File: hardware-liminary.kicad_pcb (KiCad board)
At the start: 2 copper layers, 149.2 x 73 mm, 55 parts, among them IC1 MCP6001T-I_OT, J3 UFL-Conn, J4 SWD, J5 Console, J6 Nema 7-Pin, K1 HL2-1CH-12S, Q1 CMBT2222A, Q2 PT204-6C, Q3 CMBT3904, SW1 SW_Push, U1 EESAMR34J18-V1_CT, U2 LD1117S33TR_SOT223

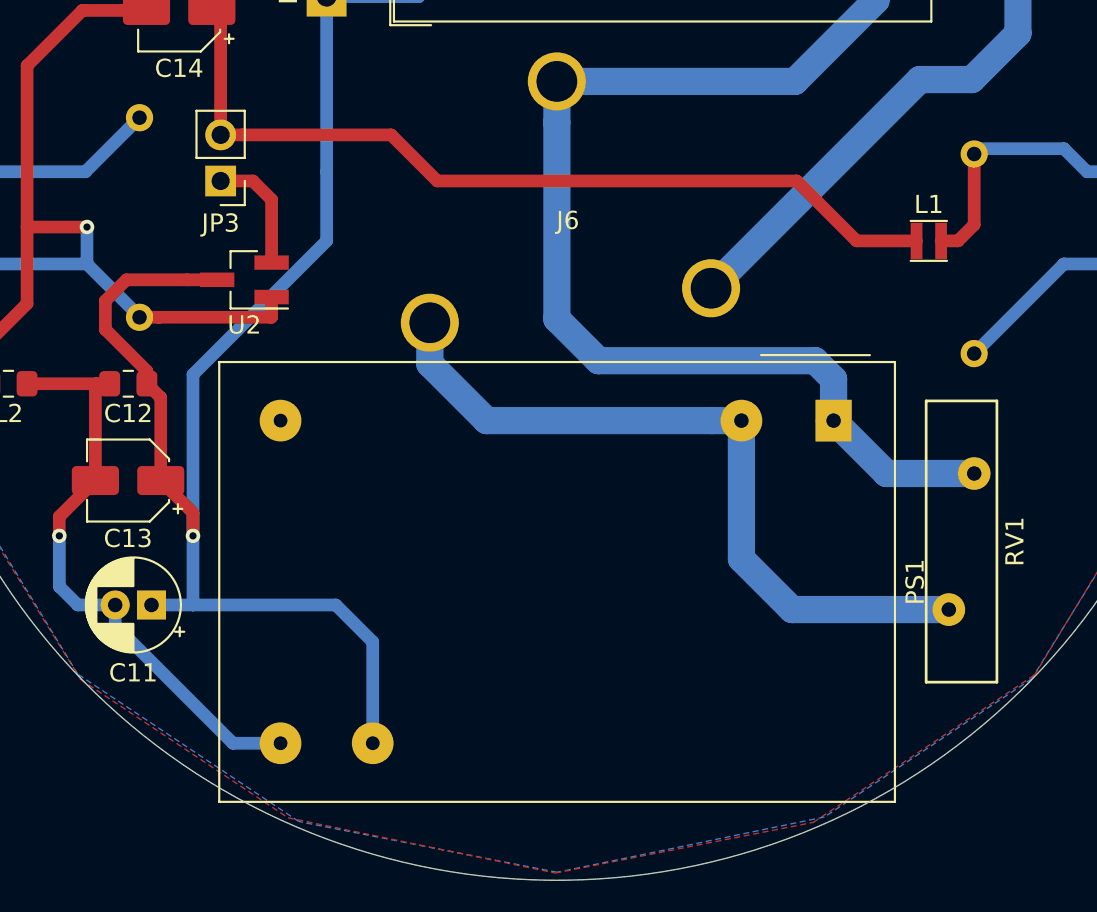
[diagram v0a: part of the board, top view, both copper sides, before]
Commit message: Correciones menores
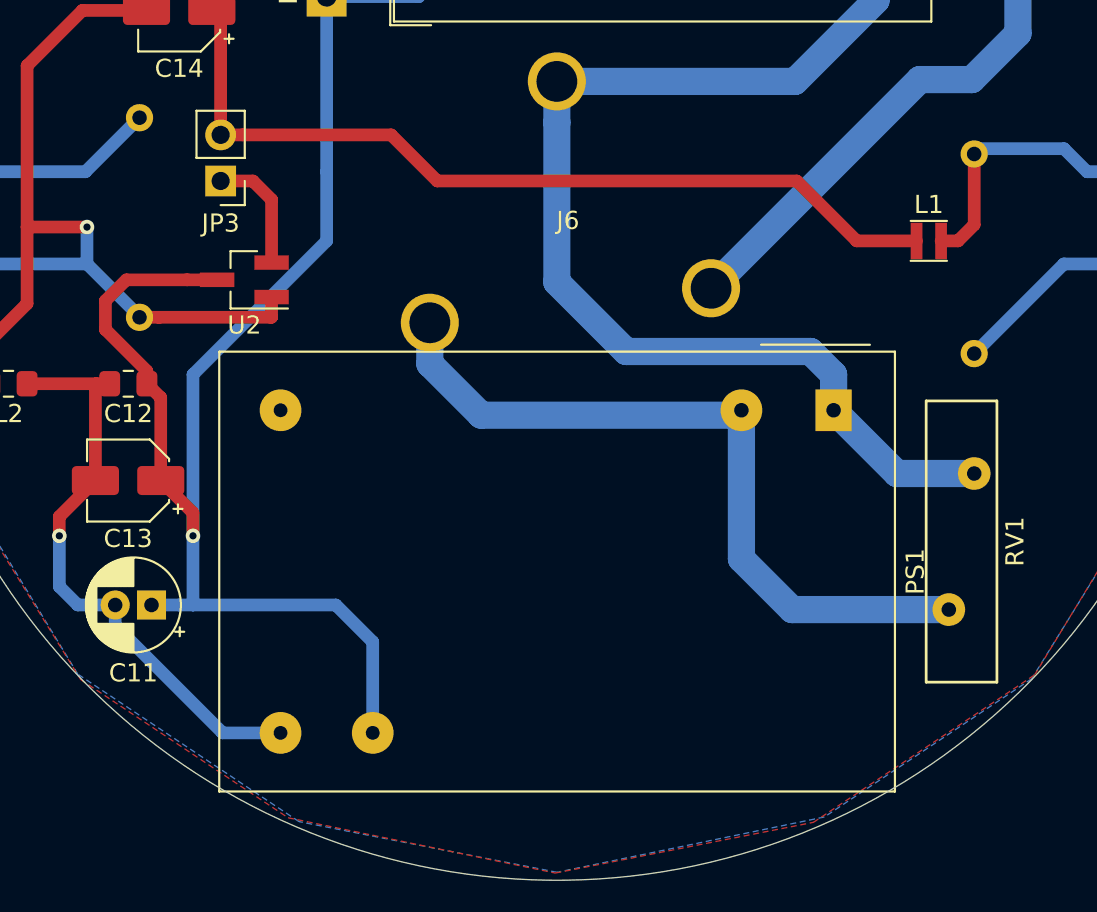
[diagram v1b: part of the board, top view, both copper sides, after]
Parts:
- moved PS1 0.57 mm to (123.4, 105.6)
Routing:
- net /Bottom Board/Linea: track 62.3 -> 60.8 mm
- net /Bottom Board/+12v: track 84.0 -> 83.5 mm
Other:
- net class Load: clearance 1.5 -> 1
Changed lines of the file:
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@@
     (thickness 1.6)
     (drawings 3)
-    (tracks 387)
+    (tracks 385)
     (zones 0)
     (modules 55)
@@
   )
   (net_class Load ""
-    (clearance 1.5)
+    (clearance 1)
     (trace_width 1.5)
     (via_dia 1.2)
@@
       (effects (font (size 1 1) (thickness 0.15)))
     )
-    (fp_circle (center 0 0) (end 36 0) (layer F.CrtYd) (width 0.12))
+    (fp_circle (center 0 0) (end 36 0) (layer Cmts.User) (width 0.12))
+    (pad 5 thru_hole circle (at -23 5.475) (size 1.5 1.5) (drill 0.8) (layers *.Cu *.Mask)
+      (net 15 GNDREF))
+    (pad 4 thru_hole circle (at -23 -5.525) (size 1.5 1.5) (drill 0.8) (layers *.Cu *.Mask)
+      (net 20 "/Bottom Board/OpenC"))
+    (pad 2 thru_hole circle (at -7 5.775) (size 3.2 3.2) (drill 2.25) (layers *.Cu *.Mask)
+      (net 31 "/Bottom Board/Neutro"))
+    (pad 1 thru_hole circle (at 0 -7.525) (size 3.2 3.2) (drill 2.25) (layers *.Cu *.Mask)
+      (net 30 "/Bottom Board/Linea"))
+    (pad 3 thru_hole circle (at 8.5 3.875) (size 3.2 3.2) (drill 2.25) (layers *.Cu *.Mask)
+      (net 29 "/Bottom Board/Carga"))
+    (pad 6 thru_hole circle (at 23 -3.525) (size 1.5 1.5) (drill 0.8) (layers *.Cu *.Mask)
+      (net 18 "/Bottom Board/3.3v"))
     (pad 7 thru_hole circle (at 23 7.475) (size 1.5 1.5) (drill 0.8) (layers *.Cu *.Mask)
       (net 19 "/Bottom Board/PIR"))
-    (pad 6 thru_hole circle (at 23 -3.525) (size 1.5 1.5) (drill 0.8) (layers *.Cu *.Mask)
-      (net 18 "/Bottom Board/3.3v"))
-    (pad 3 thru_hole circle (at 8.5 3.875) (size 3.2 3.2) (drill 2.25) (layers *.Cu *.Mask)
-      (net 29 "/Bottom Board/Carga"))
-    (pad 1 thru_hole circle (at 0 -7.525) (size 3.2 3.2) (drill 2.25) (layers *.Cu *.Mask)
-      (net 30 "/Bottom Board/Linea"))
-    (pad 2 thru_hole circle (at -7 5.775) (size 3.2 3.2) (drill 2.25) (layers *.Cu *.Mask)
-      (net 31 "/Bottom Board/Neutro"))
-    (pad 4 thru_hole circle (at -23 -5.525) (size 1.5 1.5) (drill 0.8) (layers *.Cu *.Mask)
-      (net 20 "/Bottom Board/OpenC"))
-    (pad 5 thru_hole circle (at -23 5.475) (size 1.5 1.5) (drill 0.8) (layers *.Cu *.Mask)
-      (net 15 GNDREF))
   )
   (module Resistor_SMD:R_1206_3216Metric_Pad1.42x1.75mm_HandSolder (layer F.Cu)
@@
   )
   (module proyect_new:Converter_ACDC_MeanWell_IRM-03-xx_THT (layer F.Cu)
-    (at 123.444 106.172 270)
+    (at 123.444 105.6005 270)
     (descr "ACDC-Converter, 3W, Meanwell, IRM-03, THT, https://www.meanwell.com/Upload/PDF/IRM-03/IRM-03-SPEC.PDF")
     (tags "ACDC-Converter 3W THT")
@@
   (segment (start 100.584 82.804) (end 102.108 81.28) (width 0.7) (layer B.Cu) (net 12))
   (segment (start 95.504 82.804) (end 100.584 82.804) (width 0.7) (layer B.Cu) (net 12))
-  (segment (start 88.138 116.332) (end 96.012 116.332) (width 0.7) (layer B.Cu) (net 12))
-  (segment (start 98.044 118.364) (end 96.012 116.332) (width 0.7) (layer B.Cu) (net 12))
-  (segment (start 98.044 123.952) (end 98.044 118.364) (width 0.7) (layer B.Cu) (net 12))
   (segment (start 95.504 92.456) (end 95.504 82.804) (width 0.7) (layer B.Cu) (net 12))
   (segment (start 95.504 96.266) (end 95.504 92.456) (width 0.7) (layer B.Cu) (net 12))
   (segment (start 88.138 112.522) (end 88.138 103.632) (width 0.7) (layer B.Cu) (net 12))
   (segment (start 88.138 103.632) (end 95.504 96.266) (width 0.7) (layer B.Cu) (net 12))
-  (segment (start 83.852 117.46337) (end 83.852 116.332) (width 0.7) (layer B.Cu) (net 13))
-  (segment (start 90.34063 123.952) (end 83.852 117.46337) (width 0.7) (layer B.Cu) (net 13))
-  (segment (start 92.964 123.952) (end 90.34063 123.952) (width 0.7) (layer B.Cu) (net 13))
+  (segment (start 98.044 123.3805) (end 98.044 118.364) (width 0.7) (layer B.Cu) (net 12))
+  (segment (start 96.012 116.332) (end 88.138 116.332) (width 0.7) (layer B.Cu) (net 12))
+  (segment (start 98.044 118.364) (end 96.012 116.332) (width 0.7) (layer B.Cu) (net 12))
   (via (at 80.772 112.522) (size 0.8) (drill 0.4) (layers F.Cu B.Cu) (net 13))
   (segment (start 80.772 111.462) (end 82.76 109.474) (width 0.7) (layer F.Cu) (net 13))
@@
   (segment (start 82.804 104.14) (end 82.76 104.184) (width 0.7) (layer F.Cu) (net 13))
   (segment (start 78.994 104.14) (end 82.804 104.14) (width 0.7) (layer F.Cu) (net 13))
+  (segment (start 83.852 117.46337) (end 83.852 116.332) (width 0.7) (layer B.Cu) (net 13))
+  (segment (start 92.964 123.3805) (end 89.76913 123.3805) (width 0.7) (layer B.Cu) (net 13))
+  (segment (start 89.76913 123.3805) (end 83.852 117.46337) (width 0.7) (layer B.Cu) (net 13))
   (segment (start 89.662 84.052) (end 89.176 83.566) (width 0.7) (layer F.Cu) (net 14))
   (segment (start 89.662 90.424) (end 89.662 84.052) (width 0.7) (layer F.Cu) (net 14))
@@
   (segment (start 131.064 87.376) (end 133.604 84.836) (width 1.5) (layer B.Cu) (net 29))
   (segment (start 128.1929 87.376) (end 131.064 87.376) (width 1.5) (layer B.Cu) (net 29))
-  (segment (start 123.19 106.2736) (end 123.19 106.1236) (width 1.5) (layer B.Cu) (net 30))
-  (segment (start 126.358 109.086) (end 123.444 106.172) (width 1.5) (layer B.Cu) (net 30))
-  (segment (start 131.194 109.086) (end 126.358 109.086) (width 1.5) (layer B.Cu) (net 30))
-  (segment (start 108.1913 89.740341) (end 108.1913 87.4776) (width 1.5) (layer B.Cu) (net 30))
-  (segment (start 110.49 102.87) (end 108.1913 100.5713) (width 1.5) (layer B.Cu) (net 30))
-  (segment (start 108.1913 100.5713) (end 108.1913 89.740341) (width 1.5) (layer B.Cu) (net 30))
-  (segment (start 123.444 106.172) (end 123.444 103.886) (width 1.5) (layer B.Cu) (net 30))
-  (segment (start 123.444 103.886) (end 122.428 102.87) (width 1.5) (layer B.Cu) (net 30))
-  (segment (start 122.428 102.87) (end 110.49 102.87) (width 1.5) (layer B.Cu) (net 30))
   (segment (start 121.3104 87.4776) (end 108.1913 87.4776) (width 1.5) (layer B.Cu) (net 30))
   (segment (start 125.7808 81.28) (end 125.7808 83.0072) (width 1.5) (layer B.Cu) (net 30))
   (segment (start 125.7808 83.0072) (end 121.3104 87.4776) (width 1.5) (layer B.Cu) (net 30))
-  (segment (start 116.737655 106.172) (end 118.364 106.172) (width 1.5) (layer B.Cu) (net 31))
-  (segment (start 101.1913 103.040341) (end 104.322959 106.172) (width 1.5) (layer B.Cu) (net 31))
-  (segment (start 104.322959 106.172) (end 116.737655 106.172) (width 1.5) (layer B.Cu) (net 31))
+  (segment (start 126.9295 109.086) (end 123.444 105.6005) (width 1.5) (layer B.Cu) (net 30))
+  (segment (start 131.194 109.086) (end 126.9295 109.086) (width 1.5) (layer B.Cu) (net 30))
+  (segment (start 123.444 103.632) (end 122.174 102.362) (width 1.5) (layer B.Cu) (net 30))
+  (segment (start 112.014 102.362) (end 108.1913 98.5393) (width 1.5) (layer B.Cu) (net 30))
+  (segment (start 123.444 105.6005) (end 123.444 103.632) (width 1.5) (layer B.Cu) (net 30))
+  (segment (start 108.1913 89.740341) (end 108.1913 87.4776) (width 1.5) (layer B.Cu) (net 30))
+  (segment (start 122.174 102.362) (end 112.014 102.362) (width 1.5) (layer B.Cu) (net 30))
+  (segment (start 108.1913 98.5393) (end 108.1913 89.740341) (width 1.5) (layer B.Cu) (net 30))
+  (segment (start 121.158 116.586) (end 129.794 116.586) (width 1.5) (layer B.Cu) (net 31))
+  (segment (start 101.1913 103.040341) (end 104.020969 105.87001) (width 1.5) (layer B.Cu) (net 31))
+  (segment (start 118.364 105.87001) (end 118.364 113.792) (width 1.5) (layer B.Cu) (net 31))
   (segment (start 101.1913 100.7776) (end 101.1913 103.040341) (width 1.5) (layer B.Cu) (net 31))
-  (segment (start 118.364 113.792) (end 118.364 106.172) (width 1.5) (layer B.Cu) (net 31))
-  (segment (start 129.794 116.586) (end 121.158 116.586) (width 1.5) (layer B.Cu) (net 31))
-  (segment (start 121.158 116.586) (end 118.364 113.792) (width 1.5) (layer B.Cu) (net 31))
+  (segment (start 104.020969 105.87001) (end 118.364 105.87001) (width 1.5) (layer B.Cu) (net 31))
+  (segment (start 118.364 113.792) (end 121.158 116.586) (width 1.5) (layer B.Cu) (net 31))
   (segment (start 207.005 109.596) (end 207.01 109.601) (width 0.7) (layer F.Cu) (net 32))
   (segment (start 200.878 109.596) (end 207.005 109.596) (width 1) (layer F.Cu) (net 32))
